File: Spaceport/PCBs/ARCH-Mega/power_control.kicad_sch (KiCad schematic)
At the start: 48 parts

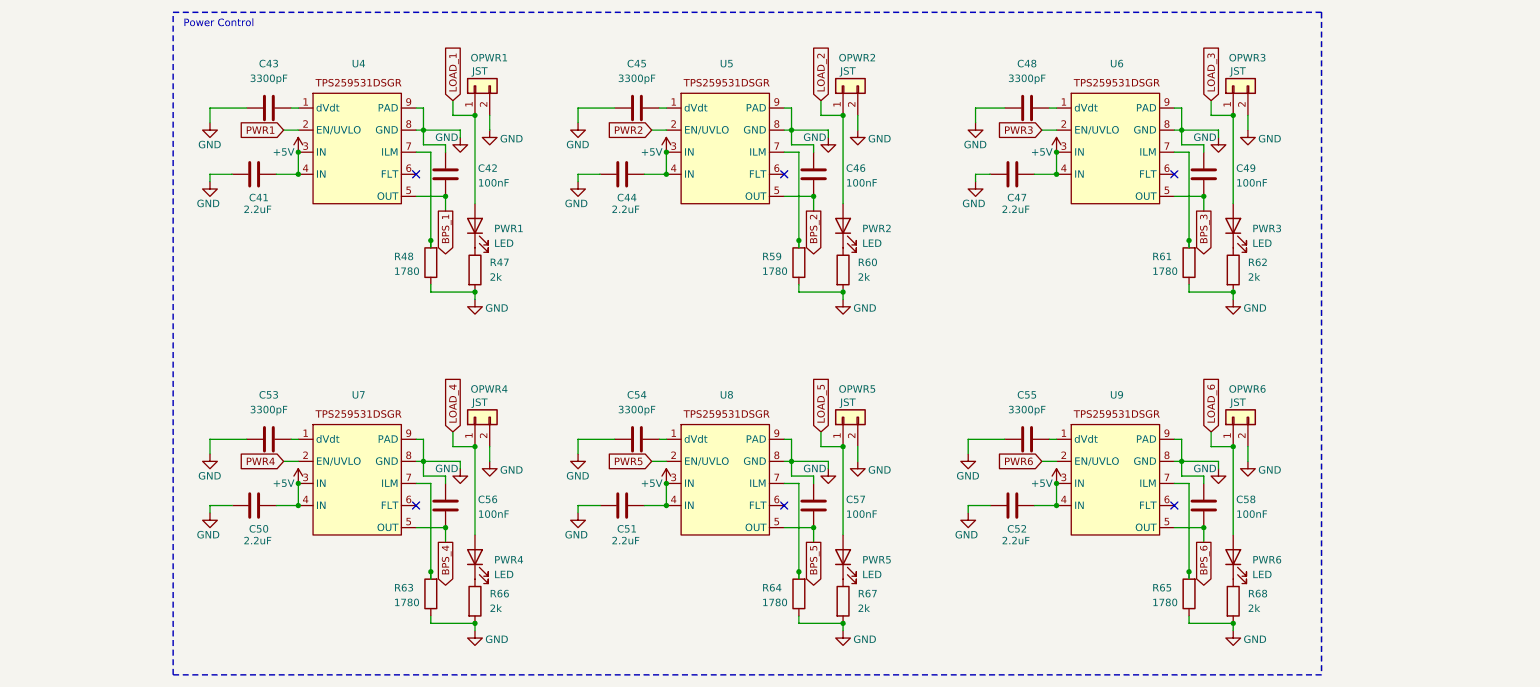
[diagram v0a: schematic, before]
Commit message: Changed capacitance values from pF to nF; Added 100k pull-down resistors to power lines; Added some space between schematic and between the cross between lines out from ILM and OUT to improve clarity.
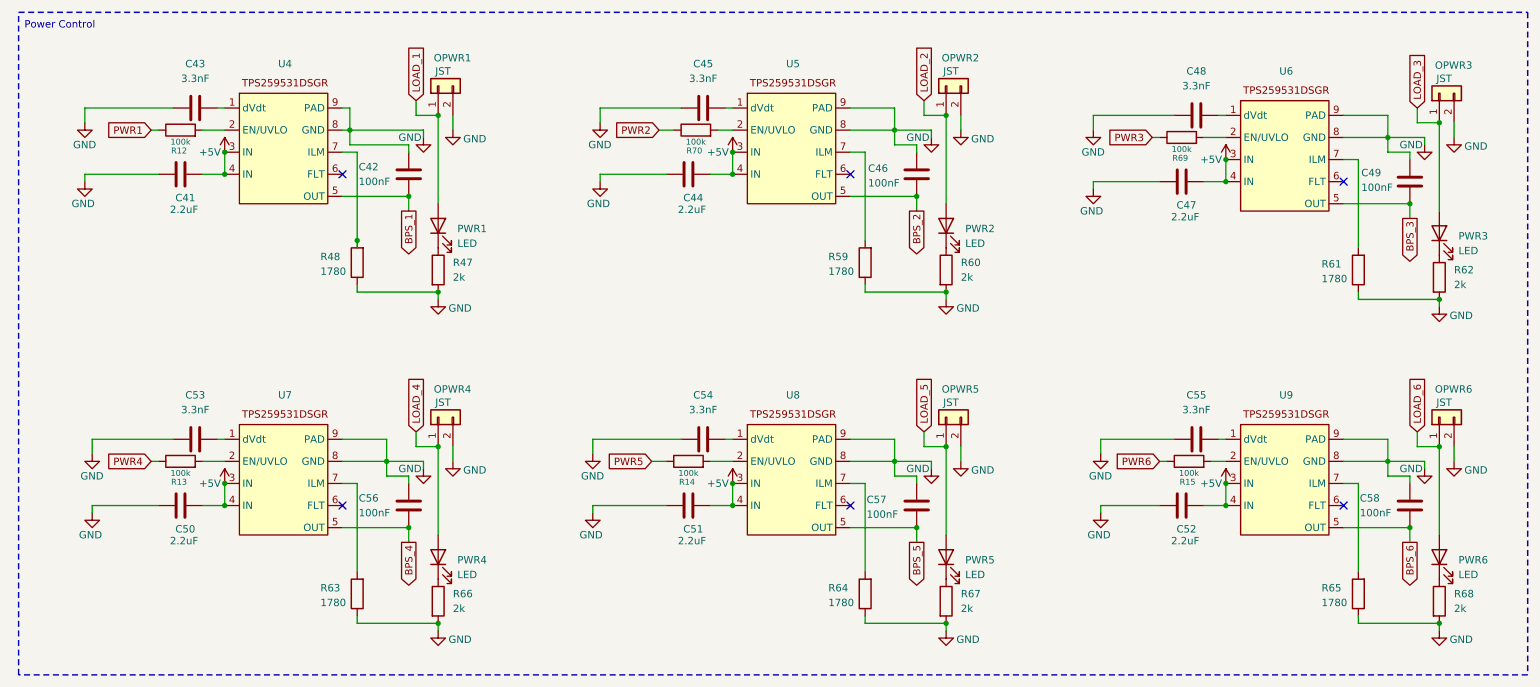
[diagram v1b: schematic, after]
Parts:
- added R12, R13, R14, R15, R69, R70: 100k, symbol Device:R
- C43, C45, C48, C53, C54, C55: value 3300pF -> 3.3nF
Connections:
- net PWR1: now also R12.1; no longer U4.2 (EN/UVLO)
- net PWR2: now also R70.1; no longer U5.2 (EN/UVLO)
- net PWR3: now also R69.1; no longer U6.2 (EN/UVLO)
- net PWR4: now also R13.1; no longer U7.2 (EN/UVLO)
- net PWR5: now also R14.1; no longer U8.2 (EN/UVLO)
- net PWR6: now also R15.1; no longer U9.2 (EN/UVLO)
- new net: R15.2, U9.2 (EN/UVLO)
- new net: R13.2, U7.2 (EN/UVLO)
- new net: R14.2, U8.2 (EN/UVLO)
- new net: R70.2, U5.2 (EN/UVLO)
- new net: R12.2, U4.2 (EN/UVLO)
- new net: R69.2, U6.2 (EN/UVLO)
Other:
- moved on the sheet: C41, C42, C43, C44, C45, C46, C47, C48, C49, C50, C51, C52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

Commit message: Added footprints and 3d models for missing components
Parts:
- C43, C45, C48, C53, C54, C55: footprint (none) -> Capacitor_SMD:C_0603_1608Metric
- OPWR1, OPWR2, OPWR3, OPWR4, OPWR5, OPWR6: footprint Avionics:JST_XH_1x2_P2.50mm_Horizontal_Small -> custom_footprints:JST_S2B-PH-K-S_LF__SN_
- R12, R13, R14, R15, R69, R70: footprint (none) -> Resistor_SMD:R_0603_1608Metric
- U4, U5, U6, U7, U8, U9: footprint (none) -> custom_footprints:SON50P200X200X80-9N
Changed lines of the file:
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@@
 			)
 		)
-		(property "Footprint" ""
+		(property "Footprint" "Resistor_SMD:R_0603_1608Metric"
 			(at 223.52 121.158 90)
 			(hide yes)
@@
 			)
 		)
-		(property "Footprint" "Avionics:JST_XH_1x2_P2.50mm_Horizontal_Small"
+		(property "Footprint" "custom_footprints:JST_S2B-PH-K-S_LF__SN_"
 			(at 266.7 111.76 0)
 			(hide yes)
@@
 			)
 		)
-		(property "Footprint" ""
+		(property "Footprint" "Capacitor_SMD:C_0603_1608Metric"
 			(at 55.88 57.4548 0)
 			(hide yes)
@@
 			)
 		)
-		(property "Footprint" ""
+		(property "Footprint" "Capacitor_SMD:C_0603_1608Metric"
 			(at 143.51 114.6048 0)
 			(hide yes)
@@
 			)
 		)
-		(property "Footprint" ""
+		(property "Footprint" "custom_footprints:SON50P200X200X80-9N"
 			(at 67.31 121.92 0)
 			(hide yes)
@@
 			)
 		)
-		(property "Footprint" "Avionics:JST_XH_1x2_P2.50mm_Horizontal_Small"
+		(property "Footprint" "custom_footprints:JST_S2B-PH-K-S_LF__SN_"
 			(at 93.98 54.61 0)
 			(hide yes)
@@
 			)
 		)
-		(property "Footprint" ""
+		(property "Footprint" "custom_footprints:SON50P200X200X80-9N"
 			(at 154.94 121.92 0)
 			(hide yes)
@@
 			)
 		)
-		(property "Footprint" "Avionics:JST_XH_1x2_P2.50mm_Horizontal_Small"
+		(property "Footprint" "custom_footprints:JST_S2B-PH-K-S_LF__SN_"
 			(at 266.7 55.88 0)
 			(hide yes)
@@
 			)
 		)
-		(property "Footprint" "Avionics:JST_XH_1x2_P2.50mm_Horizontal_Small"
+		(property "Footprint" "custom_footprints:JST_S2B-PH-K-S_LF__SN_"
 			(at 181.61 111.76 0)
 			(hide yes)
@@
 			)
 		)
-		(property "Footprint" ""
+		(property "Footprint" "custom_footprints:SON50P200X200X80-9N"
 			(at 154.94 64.77 0)
 			(hide yes)
@@
 			)
 		)
-		(property "Footprint" ""
+		(property "Footprint" "Capacitor_SMD:C_0603_1608Metric"
 			(at 143.51 57.4548 0)
 			(hide yes)
@@
 			)
 		)
-		(property "Footprint" ""
+		(property "Footprint" "Resistor_SMD:R_0603_1608Metric"
 			(at 137.16 121.158 90)
 			(hide yes)
@@
 			)
 		)
-		(property "Footprint" ""
+		(property "Footprint" "custom_footprints:SON50P200X200X80-9N"
 			(at 67.31 64.77 0)
 			(hide yes)
@@
 			)
 		)
-		(property "Footprint" ""
+		(property "Footprint" "custom_footprints:SON50P200X200X80-9N"
 			(at 240.03 121.92 0)
 			(hide yes)
@@
 			)
 		)
-		(property "Footprint" ""
+		(property "Footprint" "Capacitor_SMD:C_0603_1608Metric"
 			(at 228.6 58.7248 0)
 			(hide yes)
@@
 			)
 		)
-		(property "Footprint" "Avionics:JST_XH_1x2_P2.50mm_Horizontal_Small"
+		(property "Footprint" "custom_footprints:JST_S2B-PH-K-S_LF__SN_"
 			(at 181.61 54.61 0)
 			(hide yes)
@@
 			)
 		)
-		(property "Footprint" ""
+		(property "Footprint" "custom_footprints:SON50P200X200X80-9N"
 			(at 240.03 66.04 0)
 			(hide yes)
@@
 			)
 		)
-		(property "Footprint" ""
+		(property "Footprint" "Resistor_SMD:R_0603_1608Metric"
 			(at 49.53 64.008 90)
 			(hide yes)
@@
 			)
 		)
-		(property "Footprint" ""
+		(property "Footprint" "Resistor_SMD:R_0603_1608Metric"
 			(at 222.25 65.278 90)
 			(hide yes)
@@
 			)
 		)
-		(property "Footprint" "Avionics:JST_XH_1x2_P2.50mm_Horizontal_Small"
+		(property "Footprint" "custom_footprints:JST_S2B-PH-K-S_LF__SN_"
 			(at 93.98 111.76 0)
 			(hide yes)
@@
 			)
 		)
-		(property "Footprint" ""
+		(property "Footprint" "Capacitor_SMD:C_0603_1608Metric"
 			(at 55.88 114.6048 0)
 			(hide yes)
@@
 			)
 		)
-		(property "Footprint" ""
+		(property "Footprint" "Capacitor_SMD:C_0603_1608Metric"
 			(at 228.6 114.6048 0)
 			(hide yes)
@@
 			)
 		)
-		(property "Footprint" ""
+		(property "Footprint" "Resistor_SMD:R_0603_1608Metric"
 			(at 49.53 121.158 90)
 			(hide yes)
@@
 			)
 		)
-		(property "Footprint" ""
+		(property "Footprint" "Resistor_SMD:R_0603_1608Metric"
 			(at 138.43 64.008 90)
 			(hide yes)
